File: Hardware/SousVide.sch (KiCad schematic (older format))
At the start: 18 parts, among them J1 ISP/PDI, SW1 SW_Push, U3 7SEGMENT_CC, U4 7SEGMENT_CC, U5 7SEGMENT_CC, U6 7SEGMENT_CC, U7 LM35-NEB

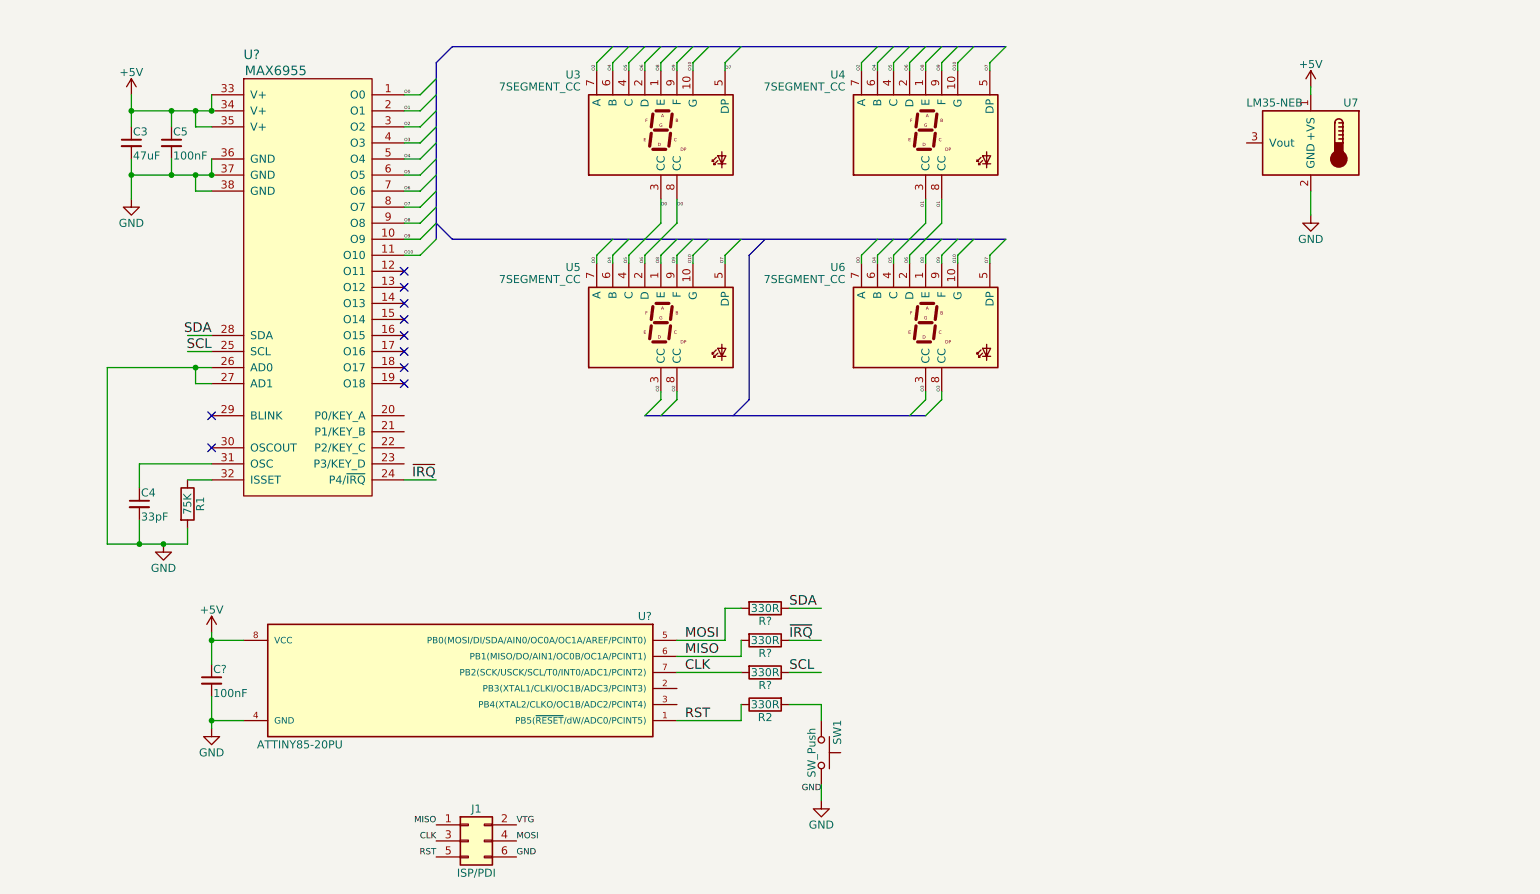
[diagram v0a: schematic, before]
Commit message: Created board layout.
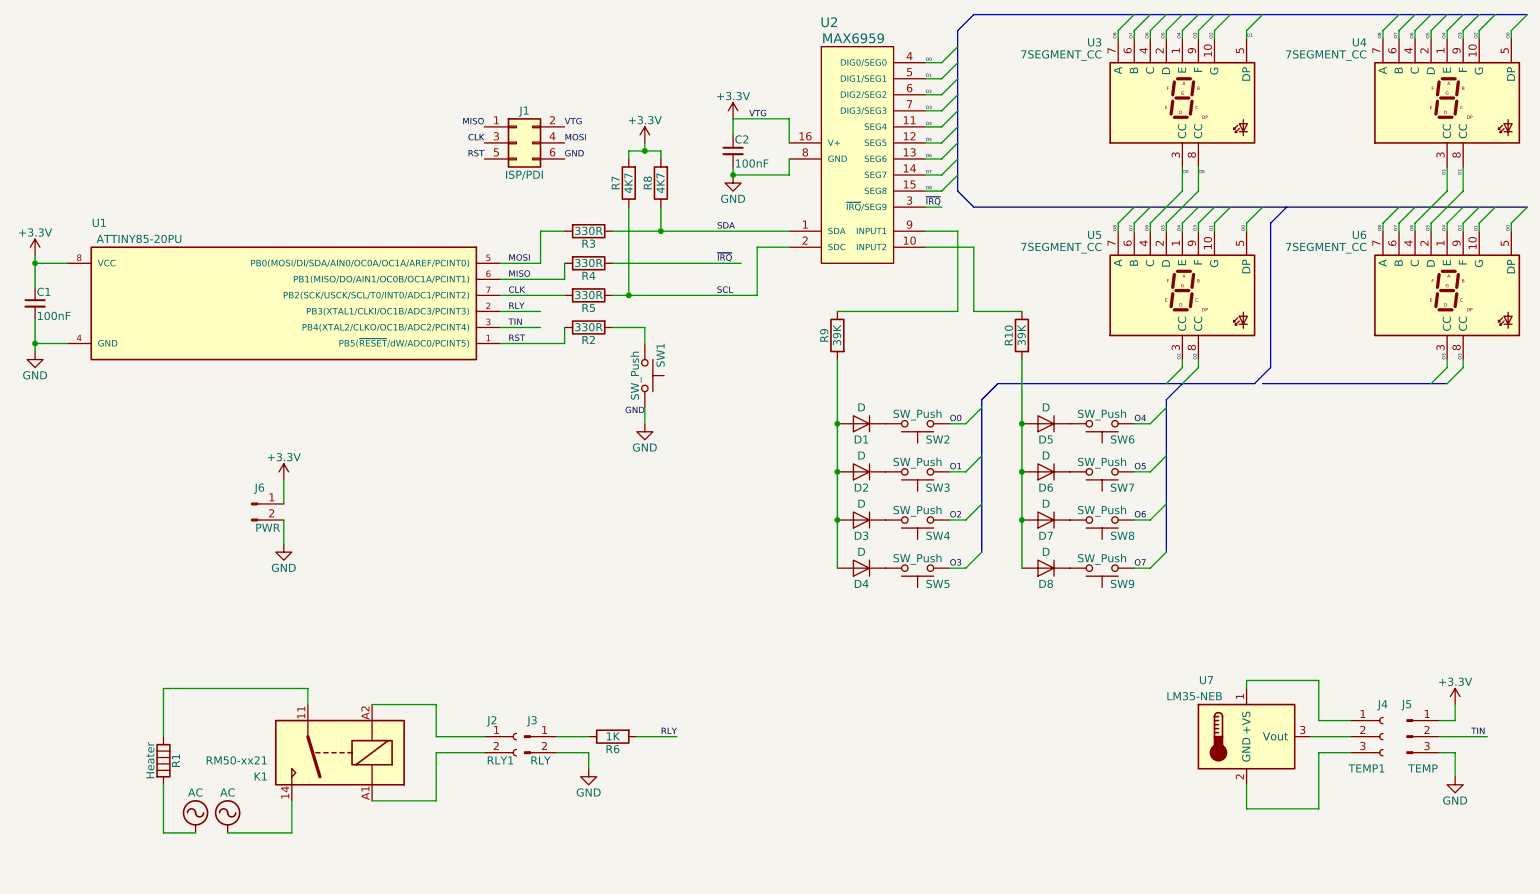
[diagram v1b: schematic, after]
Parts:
- removed C3: 47uF, symbol C_Small
- removed C4: 33pF, symbol C_Small
- removed C5: 100nF, symbol C_Small
- removed R1: 75K, symbol R
- removed U?: MAX6955, symbol MAX6955
- added C2: 100nF, Capacitors_THT:C_Disc_D3.8mm_W2.6mm_P2.50mm, symbol C_Small
- added D1, D2, D3, D4, D5, D6, D7, D8: D, Diodes_THT:D_DO-35_SOD27_P7.62mm_Horizontal, symbol D
- added J2: RLY1, symbol Conn_01x02_Female
- added J3: RLY, Pin_Headers:Pin_Header_Straight_1x02_Pitch2.54mm, symbol Conn_01x02_Male
- added J4: TEMP1, symbol Conn_01x03_Female
- added J5: TEMP, Pin_Headers:Pin_Header_Straight_1x03_Pitch2.54mm, symbol Conn_01x03_Male
- added J6: PWR, Pin_Headers:Pin_Header_Straight_1x02_Pitch2.54mm, symbol Conn_01x02_Male
- added K1: RM50-xx21, symbol RM50-xx21
- added R1: Heater, symbol Heater
- added R10, R9: 39K, Resistors_THT:R_Axial_DIN0207_L6.3mm_D2.5mm_P7.62mm_Horizontal, symbol R
- added R6: 1K, Resistors_THT:R_Axial_DIN0207_L6.3mm_D2.5mm_P7.62mm_Horizontal, symbol R
- added R7, R8: 4K7, Resistors_THT:R_Axial_DIN0207_L6.3mm_D2.5mm_P7.62mm_Horizontal, symbol R
- added SW2, SW3, SW4, SW5, SW6, SW7, SW8, SW9: SW_Push, Buttons_Switches_THT:SW_TH_Tactile_Omron_B3F-10xx, symbol SW_Push
- added U2: MAX6959, Housings_DIP:DIP-16_W7.62mm, symbol MAX6959
- C1: renamed from C?; footprint (none) -> Capacitors_THT:C_Disc_D3.8mm_W2.6mm_P2.50mm
- J1: footprint (none) -> Pin_Headers:Pin_Header_Straight_2x03_Pitch2.54mm
- R2: footprint (none) -> Resistors_THT:R_Axial_DIN0207_L6.3mm_D2.5mm_P7.62mm_Horizontal
- R3, R4, R5: renamed from R?; footprint (none) -> Resistors_THT:R_Axial_DIN0207_L6.3mm_D2.5mm_P7.62mm_Horizontal
- SW1: footprint (none) -> Buttons_Switches_THT:SW_TH_Tactile_Omron_B3F-10xx
- U3, U4, U5, U6: footprint (none) -> Displays_7-Segment:7SegmentLED_LTS6760_LTS6780
- gave numbers to parts that had none: 1
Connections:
- net labels added: +3.3V, AC, RLY, TIN
- net labels removed: +5V, O10, O9
- wire segments 96 -> 133
- no-connect marks 10 -> 0
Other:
- moved on the sheet: C1, J1, R2, R3, R4, R5, SW1, U1, U3, U4, U5, U6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
